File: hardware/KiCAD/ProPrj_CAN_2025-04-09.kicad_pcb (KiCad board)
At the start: 2 copper layers, 27.8 x 40.4 mm, 20 parts

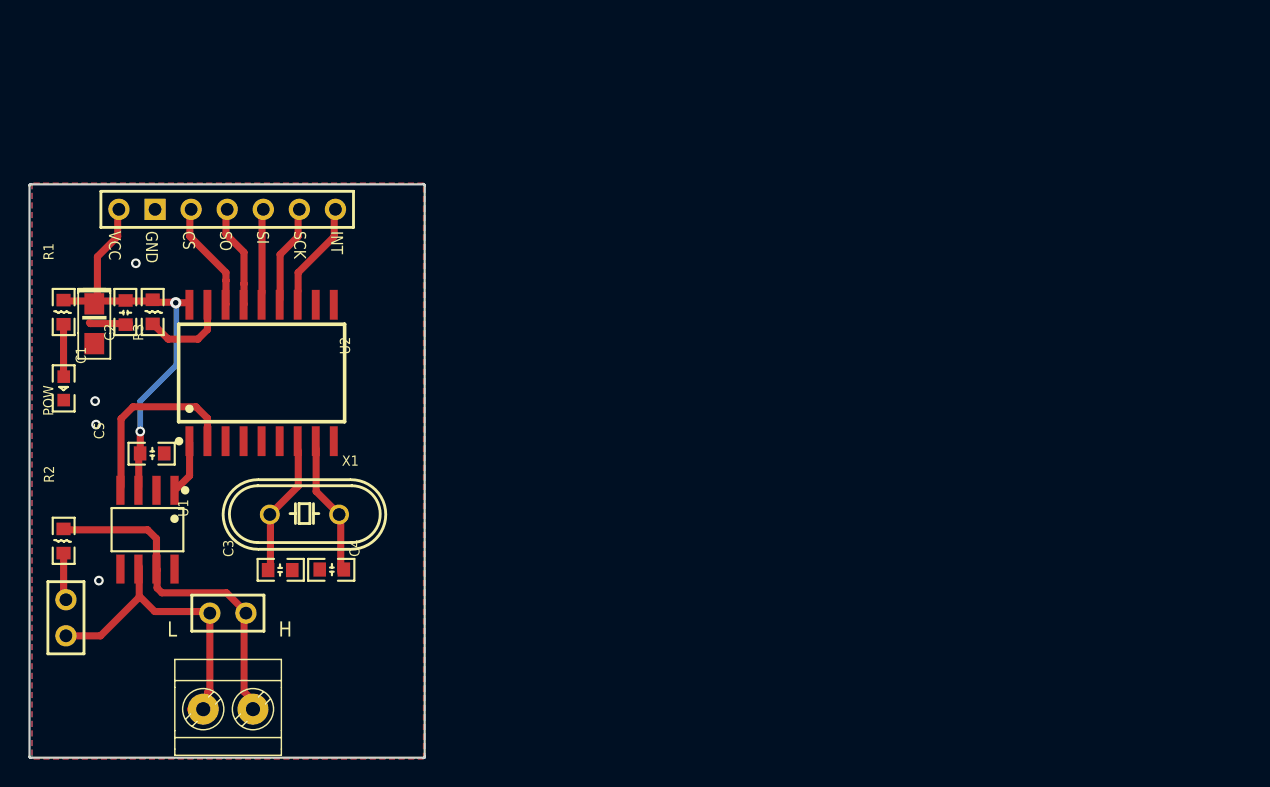
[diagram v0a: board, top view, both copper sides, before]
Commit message: edit
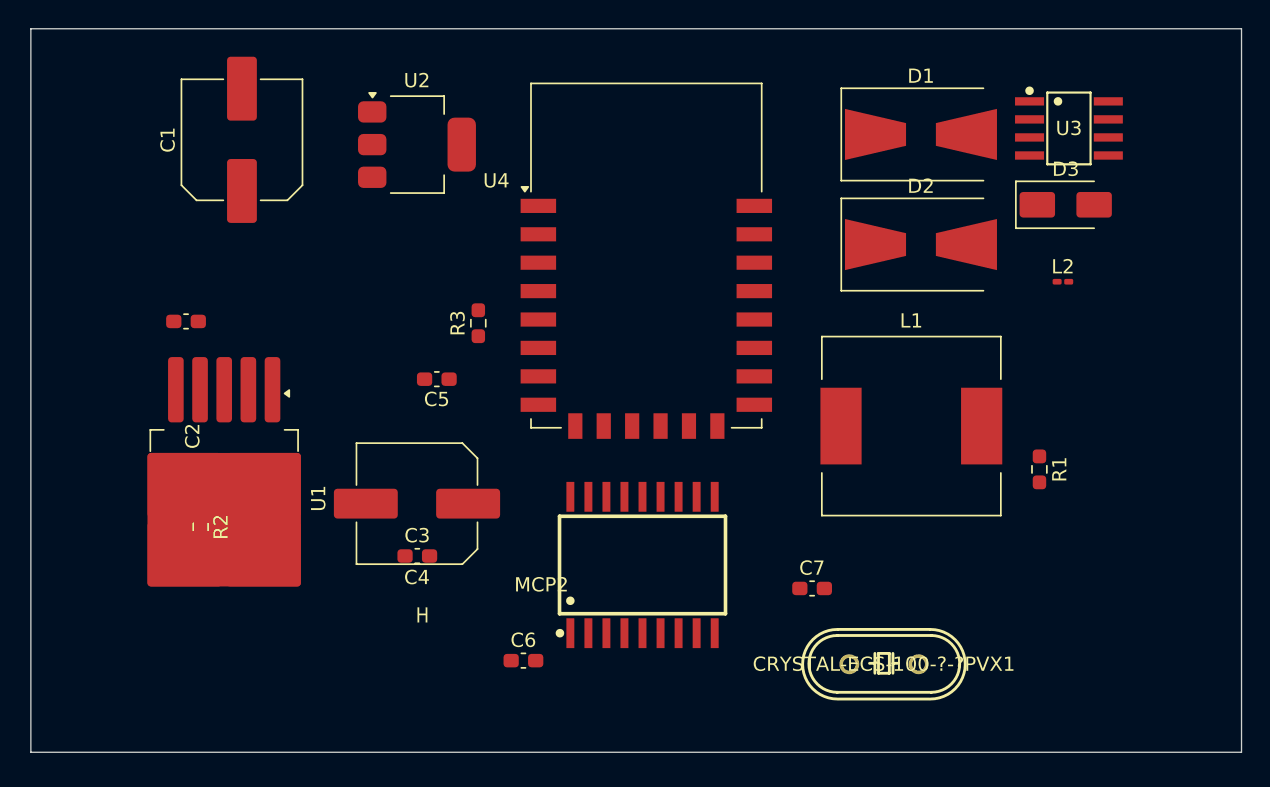
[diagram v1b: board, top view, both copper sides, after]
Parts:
- removed ?: , ProPrj_CAN_2025-04-09:Pad_ie6
- removed ?: , ProPrj_CAN_2025-04-09:Pad_ie7
- removed ?: , ProPrj_CAN_2025-04-09:Pad_ie5
- removed ?: , ProPrj_CAN_2025-04-09:Pad_ie8
- removed P1: , ProPrj_CAN_2025-04-09:HDR1X7
- removed P2, P3: , ProPrj_CAN_2025-04-09:HDR1X2
- removed P4: , ProPrj_CAN_2025-04-09:TERMINAL-BLOCK-2-PIN-3.5MM-ROUND-PAD
- removed POW: , ProPrj_CAN_2025-04-09:CHIPLED_0603
- removed X1: , ProPrj_CAN_2025-04-09:HC-49US_L11.5-W4.5-P4.88
- added C6: 22 pF, Capacitor_SMD:C_0603_1608Metric_Pad1.08x0.95mm_HandSolder, F.Cu at (164.6, 123.3)
- added C7: 22 pF, Capacitor_SMD:C_0603_1608Metric_Pad1.08x0.95mm_HandSolder, F.Cu at (184.9, 118.3)
- added CRYSTAL-ECS-100-?-?PVX1: 8MHz, ProPrj_CAN_2025-04-09:HC-49US_L11.5-W4.5-P4.88, F.Cu at (190.0, 123.6)
- added D1: SS510C, Diode_SMD:D_SMB-SMC_Universal_Handsoldering, F.Cu at (192.6, 86.3)
- added D2: SS510C, Diode_SMD:D_SMB-SMC_Universal_Handsoldering, F.Cu at (192.6, 94.1)
- added D3: SMAJ33CA, Diode_SMD:D_SMA, F.Cu at (202.8, 91.3)
- added L1: 100 uH, Inductor_SMD:L_12x12mm_H8mm, F.Cu at (191.9, 106.8)
- added L2: BLM18PG121SN1D, Inductor_SMD:L_0201_0603Metric_Pad0.64x0.40mm_HandSolder, F.Cu at (202.6, 96.7)
- added MCP2: MCP2515-I, ProPrj_CAN_2025-04-09:SOIC-18_L11.6-W7.5-P1.27-LS10.3-BL, F.Cu at (173.0, 116.6)
- added U3: TJA1050DRG, ProPrj_CAN_2025-04-09:SOIC-8E, F.Cu at (203.0, 85.9)
- added U4: ESP-12F, RF_Module:ESP-12E, F.Cu at (173.2, 94.8)
- C1: value (none) -> 470 uF; footprint ProPrj_CAN_2025-04-09:tantalum A -> Capacitor_SMD:C_Elec_8x10.2
- C2, C3, C5: value (none) -> 100 nF; footprint ProPrj_CAN_2025-04-09:C0603 -> Capacitor_SMD:C_0603_1608Metric_Pad1.08x0.95mm_HandSolder
- C4: value (none) -> 470 uF; footprint ProPrj_CAN_2025-04-09:C0603 -> Capacitor_SMD:C_Elec_8x10.2
- R1, R2, R3: value (none) -> 10 k; footprint ProPrj_CAN_2025-04-09:R0603 -> Resistor_SMD:R_0603_1608Metric_Pad0.98x0.95mm_HandSolder
- U1: value (none) -> LM2575-5.0BT; footprint ProPrj_CAN_2025-04-09:SOIC-8E -> Package_TO_SOT_SMD:TO-263-5_TabPin3
- U2: value (none) -> AMS1117-3.3; footprint ProPrj_CAN_2025-04-09:SOIC-18_L11.6-W7.5-P1.27-LS10.3-BL -> Package_TO_SOT_SMD:SOT-223-3_TabPin2
- moved R1 69.6 mm to (200.9, 109.9)
- moved R3 22.9 mm to (161.4, 99.6)
- moved C5 20.7 mm to (158.5, 103.5)
- moved U2 19.4 mm to (157.1, 87.0)
- moved C1 16.6 mm to (144.8, 86.7), turned to 90 degrees
- moved C3 9.70 mm to (157.1, 116.0)
- moved R2 9.70 mm to (141.9, 113.9)
- moved C4 7.58 mm to (157.1, 112.3)
- moved U1 5.83 mm to (143.5, 111.9)
- moved C2 4.30 mm to (140.8, 99.5), turned to 180 degrees
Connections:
- C1 pad 1: (no net) -> VCC
- C1 pad 2: (no net) -> GND
- C2 pad 1: (no net) -> VCC
- C2 pad 2: (no net) -> GND
- C3 pad 1: (no net) -> VCC
- C3 pad 2: (no net) -> GND
- C4 pad 1: (no net) -> Net-(D2-K)
- C4 pad 2: (no net) -> GND
- C5 pad 1: (no net) -> Net-(D2-K)
- C5 pad 2: (no net) -> GND
- R1 pad 1: (no net) -> VCC
- R1 pad 2: (no net) -> Net-(MCP2-~RESET~)
- R2 pad 1: (no net) -> Net-(J1-Pin_1)
- R2 pad 2: (no net) -> Net-(U3-CANH)
- R3 pad 1: (no net) -> +3.3V
- R3 pad 2: (no net) -> Net-(U4-EN)
- U1 pad 1: (no net) -> Net-(D2-K)
- U1 pad 2: (no net) -> Net-(D1-K)
- U1 pad 3: (no net) -> GND
- U1 pad 4: (no net) -> VCC
- U1 pad 5: (no net) -> GND
- U2 pad 1: (no net) -> GND
- U2 pad 2: (no net) -> +3.3V
- U2 pad 3: (no net) -> VCC
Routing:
- net 0: track 160.7 -> 0.00 mm, vias 6 -> 0
- removed copper zone on B.Cu, net (none)
- removed copper zone on F.Cu, net (none)
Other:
- board size 27.8 x 40.4 mm -> 85.2 x 50.9 mm
- board text removed: "CAN Bus Module"
- board text removed: "CS"
- board text removed: "GND"
- board text removed: "INT"
- board text removed: "L"
- board text removed: "SCK"
- board text removed: "SI"
- board text removed: "SO"
- board text removed: "VCC"
